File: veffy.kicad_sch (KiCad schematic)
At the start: 91 parts, among them J1 SWD, Q1 2N7002, Q2 BFR93A, Q3 2N7002, Q4 BFR93AE6327HTSA1, SW1 SW_Push, U1 ATSAMD21G18A-A, U2 ADF4112BCPZ, U3 SA612AN/01_112, U4 MC3361, U5 LM386, U6 LM358_DFN, U7 AD9834, U8 QPA9510, Y2 TCXO-14

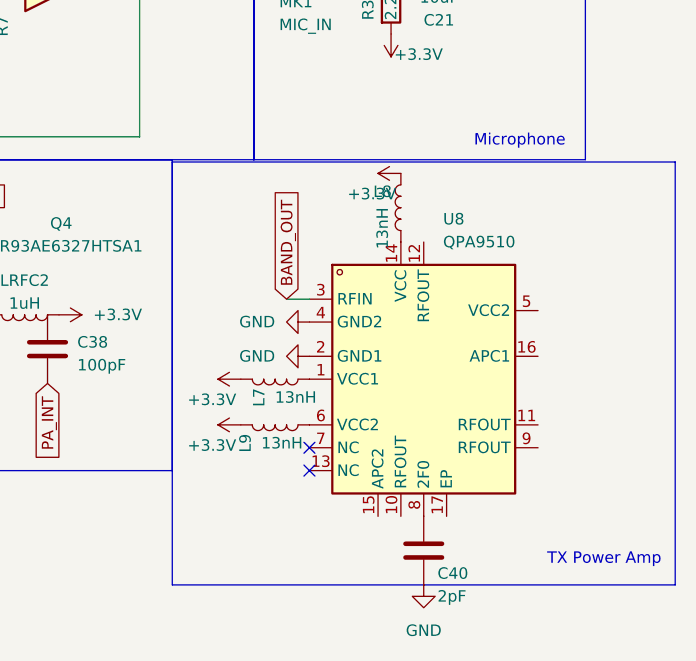
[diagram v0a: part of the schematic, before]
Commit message: almost done the power amp
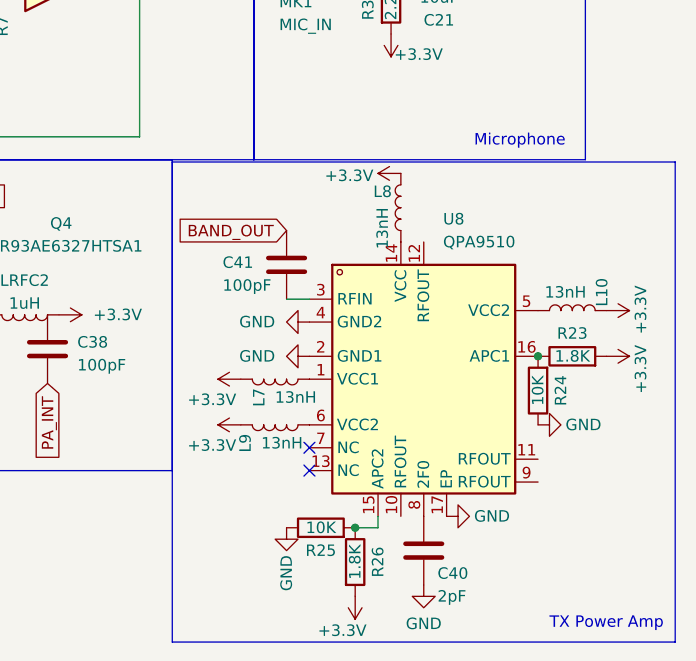
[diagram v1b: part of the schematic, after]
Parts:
- added C41: 100pF, Capacitor_SMD:C_0603_1608Metric, symbol Device:C
- added L10: 13nH, Inductor_SMD:L_0603_1608Metric, symbol Device:L
- added R23, R26: 1.8K, symbol Device:R
- added R24, R25: 10K, symbol Device:R
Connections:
- net +3.3V: now also L10.2, R23.2, R26.2
- net BAND_OUT: now also C41.1; no longer U8.3 (RFIN)
- net GND: now also U8.17 (EP), R24.1, R25.1
- net at U8.15 (APC2): now also R25.2, R26.1
- net at U8.16 (APC1): now also R23.1, R24.2
- net at U8.5 (VCC2): now also L10.1
- new net: C41.2, U8.3 (RFIN)
